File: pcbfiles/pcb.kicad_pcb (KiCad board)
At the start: 2 copper layers, 269.9 x 139.7 mm, 256 parts, among them J1 Conn_01x06, J2 Conn_01x06, J3 Conn_01x06, J4 Conn_01x06, J5 Conn_01x04_Female, J6 Conn_01x04_Female, Q1 AO3401A, Q2 AO3401A, SW1 SW_SPST, SW10 SW_SPST, SW11 SW_SPST, SW12 SW_SPST, SW13 SW_SPST, SW14 SW_SPST, SW15 SW_SPST, SW16 SW_SPST, SW17 SW_SPST, SW18 SW_SPST, SW19 SW_SPST, SW2 SW_SPST, SW20 SW_SPST, SW21 SW_SPST, SW22 SW_SPST, SW23 SW_SPST, SW24 SW_SPST, SW25 SW_SPST, SW26 SW_SPST, SW27 SW_SPST, SW28 SW_SPST, SW29 SW_SPST, SW3 SW_SPST, SW30 SW_SPST, SW31 SW_SPST, SW32 SW_SPST, SW33 SW_SPST, SW34 SW_SPST, SW35 SW_SPST, SW36 SW_SPST, SW37 SW_SPST, SW38 SW_SPST, SW39 SW_SPST, SW4 SW_SPST, SW40 SW_SPST, SW41 SW_SPST, SW42 SW_SPST, SW43 SW_SPST, SW44 SW_SPST, SW45 SW_SPST, SW46 SW_SPST, SW47 SW_SPST, SW48 SW_SPST, SW49 SW_SPST, SW5 SW_SPST, SW50 SW_SPST, SW51 SW_SPST, SW52 SW_SPST, SW53 SW_SPST, SW54 SW_SPST, SW55 SW_SPST, SW56 SW_SPST, SW57 SW_SPST, SW58 SW_SPST, SW59 SW_SPST, SW6 SW_SPST, SW60 SW_SPST, SW61 SW_SPST, SW62 SW_SPST, SW63 SW_SPST, SW64 SW_SPST, SW65 SW_SPST, SW66 SW_SPST, SW67 SW_SPST, SW68 SW_SPST, SW69 SW_SPST, SW7 SW_SPST, SW70 SW_SPST, SW71 SW_SPST, SW72 SW_SPST, SW73 SW_SPST, SW74 SW_SPST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

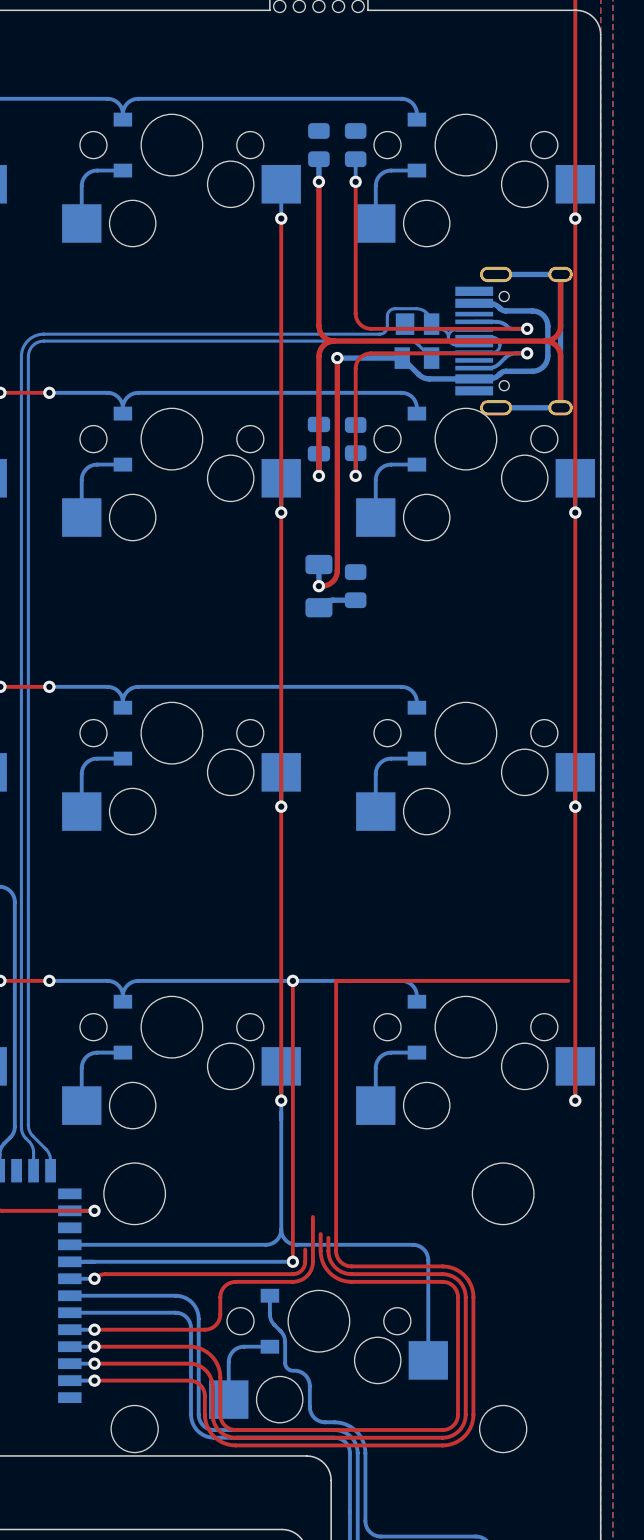
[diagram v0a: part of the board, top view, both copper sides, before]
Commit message: Routing
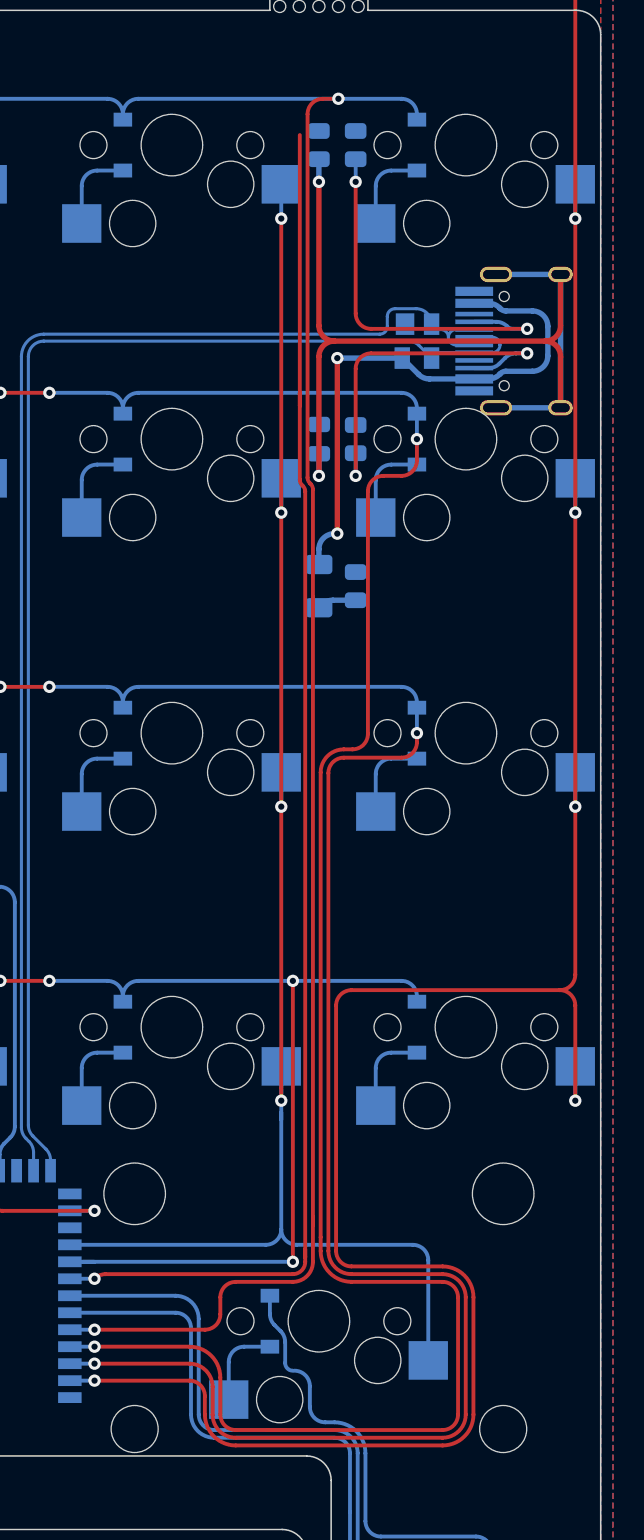
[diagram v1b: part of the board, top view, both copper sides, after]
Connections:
- U6 pad 30: unconnected-(U6-Pad30) -> RH_COL4
- U6 pad 33: unconnected-(U6-Pad33) -> RH_ROW1
- U6 pad 34: unconnected-(U6-Pad34) -> RH_ROW2
- U6 pad 35: unconnected-(U6-Pad35) -> RH_ROW3
- U6 pad 36: unconnected-(U6-Pad36) -> RH_COL6
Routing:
- net RH_ROW2: track 124.9 -> 232.2 mm, vias 2 -> 4
- net RH_ROW1: track 111.4 -> 208.2 mm, vias 0 -> 2
- net RH_COL4: track 83.5 -> 173.7 mm, vias 6 -> 7
- net RH_ROW3: track 136.0 -> 223.9 mm, vias 4 -> 6
- net unconnected-(U6-Pad36): track 80.6 -> 0.00 mm, vias 1 -> 0
- net RH_COL6: track 87.3 -> 167.4 mm, vias 5 -> 6
- net unconnected-(U6-Pad34): track 50.0 -> 0.00 mm, vias 1 -> 0
- net unconnected-(U6-Pad35): track 48.8 -> 0.00 mm, vias 1 -> 0
- net unconnected-(U6-Pad33): track 21.5 -> 0.00 mm, vias 1 -> 0
- net unconnected-(U6-Pad30): track 16.6 -> 0.00 mm, vias 1 -> 0
- net RAW_B: track 39.1 -> 36.3 mm

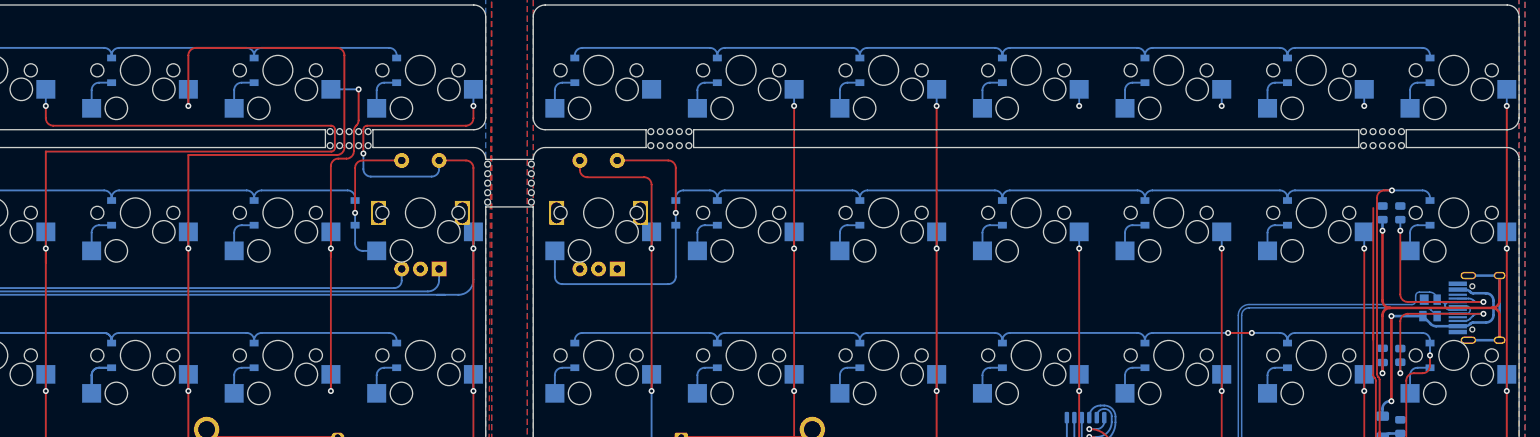
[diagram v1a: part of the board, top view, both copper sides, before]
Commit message: Routing.
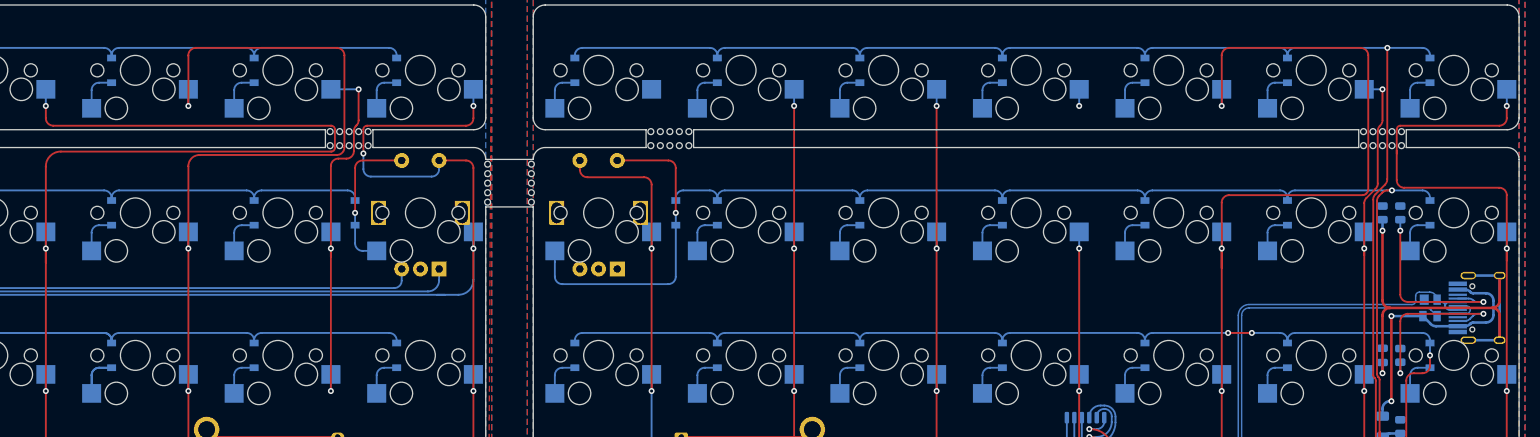
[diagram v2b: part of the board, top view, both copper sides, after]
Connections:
- U6 pad 30: RH_COL4 -> RH_ROW0
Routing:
- net RH_ROW0: track 124.9 -> 236.3 mm, vias 0 -> 2
- net RH_COL6: track 167.4 -> 197.1 mm
- net RH_COL5: track 108.4 -> 131.7 mm
- net RH_COL4: track 173.7 -> 158.1 mm, vias 7 -> 6
- net LH_COL3: track 231.7 -> 230.7 mm
- net LH_COL4: track 252.4 -> 251.7 mm
